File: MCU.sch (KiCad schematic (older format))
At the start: 36 parts, among them P1 CONN_02X05, P2 USB_OTG, SW48 Reset, U1 IS31FL3732, U2 MK20DX256VLH7, X1 CRYSTAL_SMD

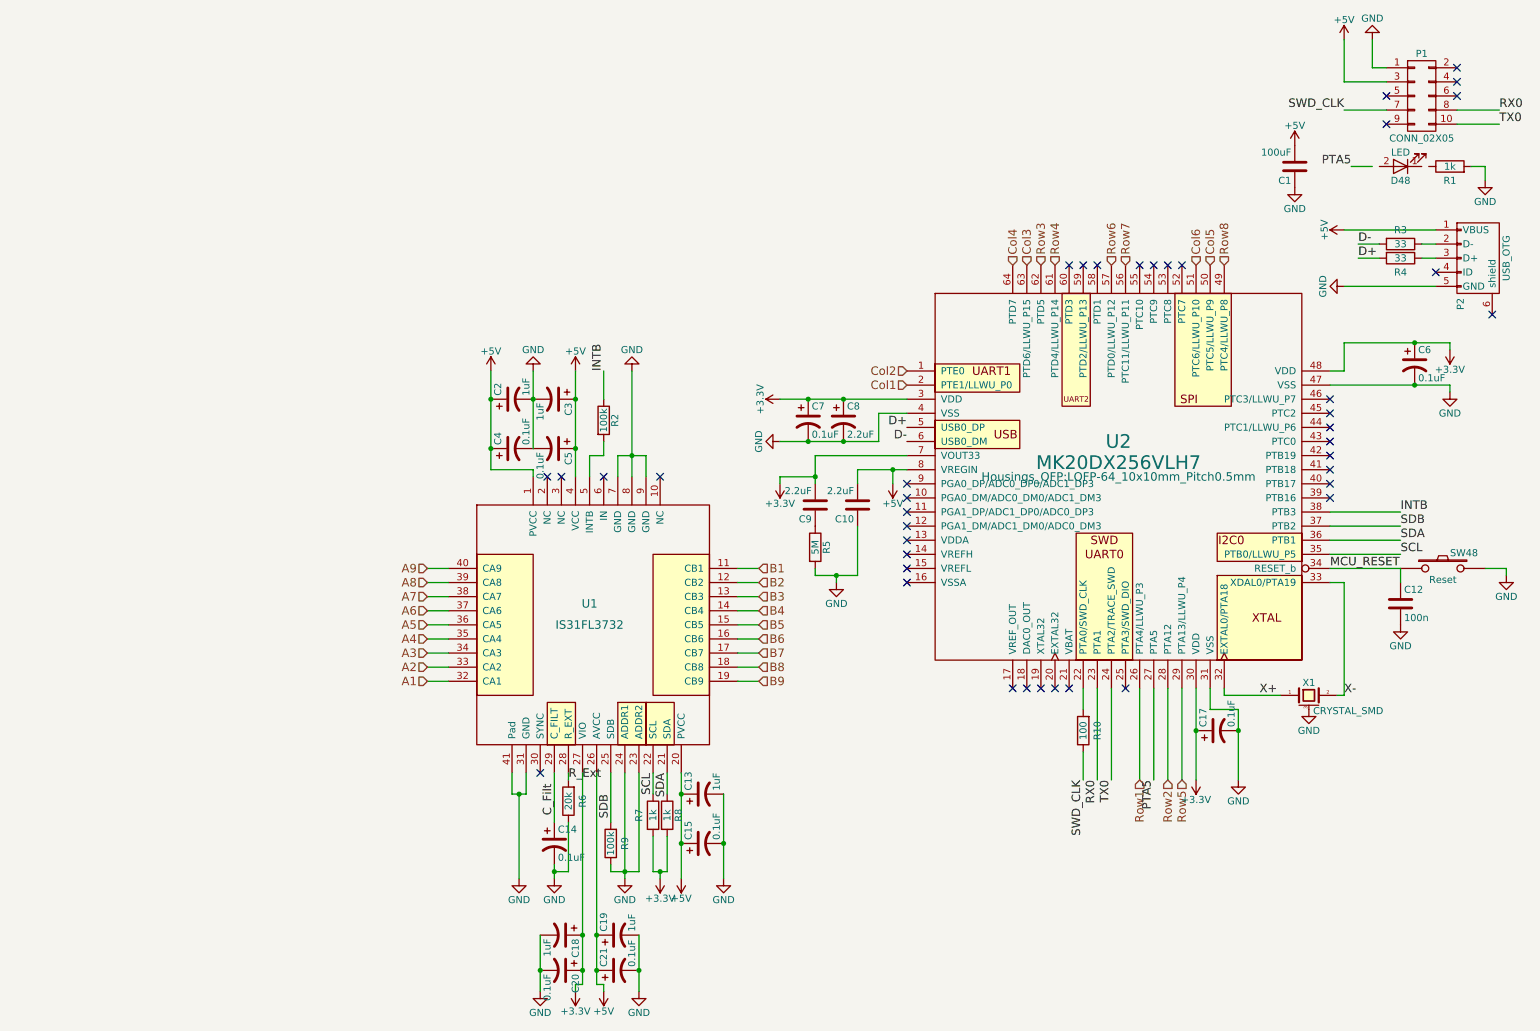
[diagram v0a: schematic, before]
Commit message: Reworked the Board
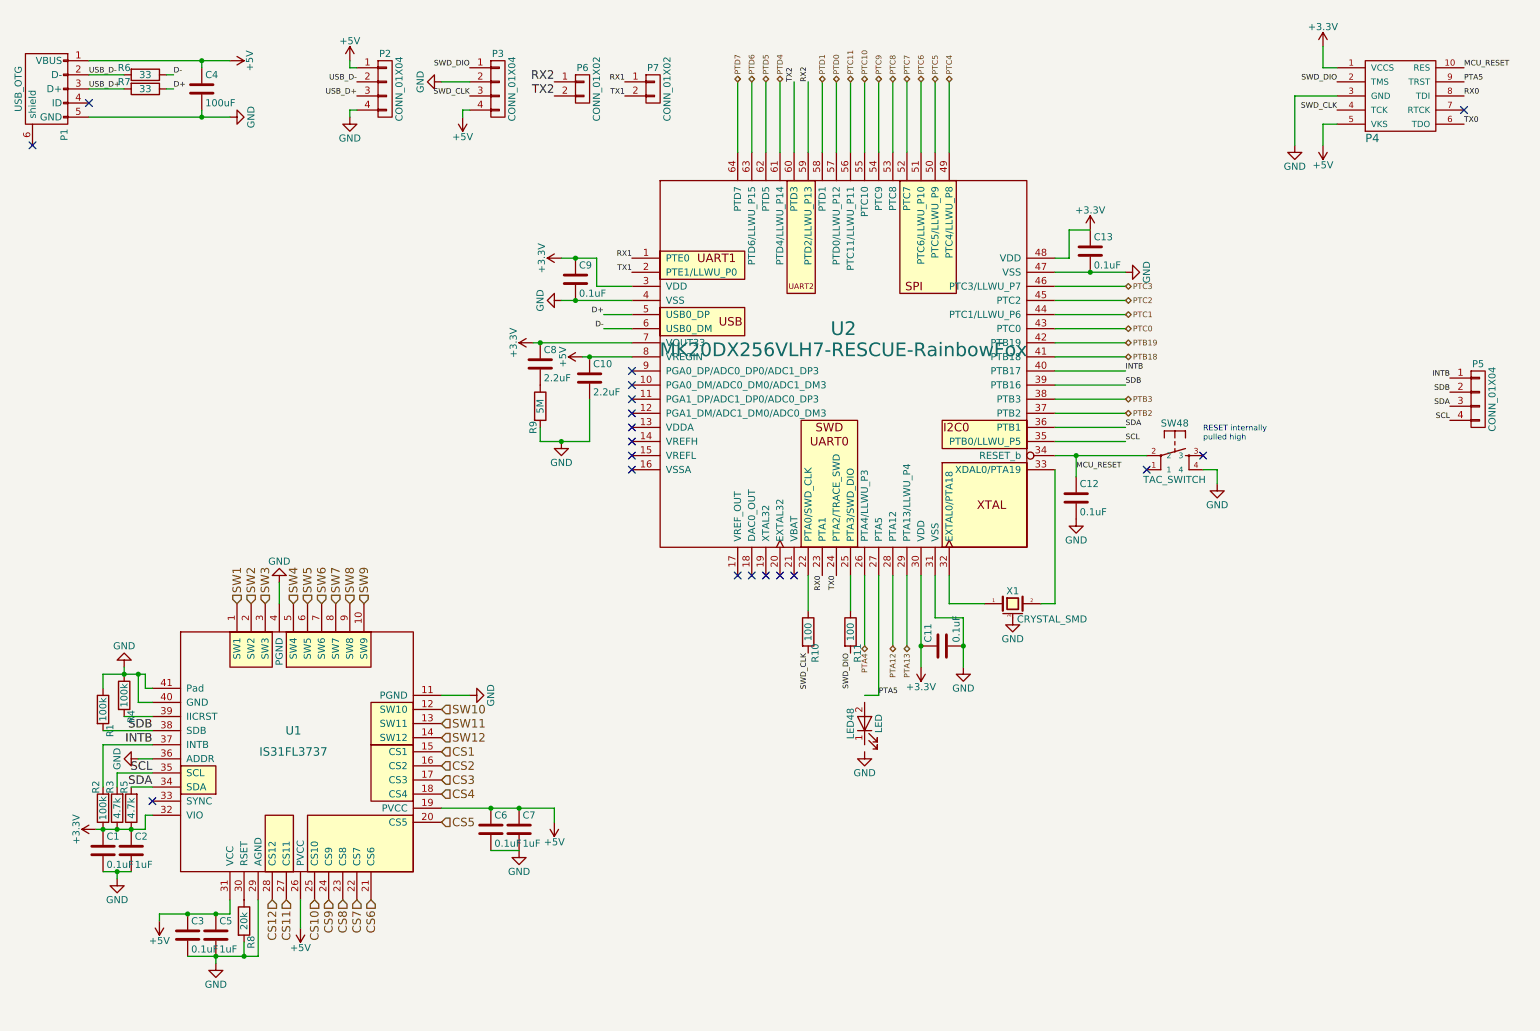
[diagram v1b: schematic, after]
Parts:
- removed C13, C18, C19, C2, C3: 1uF, Capacitors_SMD:C_0603, symbol CP1
- removed C14, C15, C17, C20, C21, C4, C5, C6, C7: 0.1uF, Capacitors_SMD:C_0603, symbol CP1
- removed C8: 2.2uF, Capacitors_SMD:C_0603, symbol CP1
- removed D48: LED, LEDs:LED_0805, symbol LED
- removed P1: CONN_02X05, Pin_Headers:Pin_Header_Straight_2x05, symbol CONN_02X05
- removed P2: USB_OTG, Connect:USB_Micro-B, symbol USB_OTG
- removed SW48: Reset, mx2a:KSEM31GLFS, symbol SW_PUSH
- removed U1: IS31FL3732, Housings_DFN_QFN:UQFN-40-1EP_5x5mm_Pitch0.4mm, symbol IS31FL3732
- removed U2: MK20DX256VLH7, Housings_QFP:LQFP-64_10x10mm_Pitch0.5mm, symbol MK20DX256VLH7
- added C11, C13, C3, C6: 0.1uF, Capacitors_SMD:C_0603, symbol C
- added C2, C5, C7: 1uF, Capacitors_SMD:C_0603, symbol C
- added C4: 100uF, Capacitors_SMD:C_1206, symbol C
- added C8: 2.2uF, Capacitors_SMD:C_0603, symbol C
- added LED48: LED, lib.pretty:LED_0805, symbol LED
- added P1: USB_OTG, lib.pretty:Micro-USB_629105150521, symbol USB_OTG
- added P2, P3, P5: CONN_01X04, lib.pretty:Conn-4, symbol CONN_01X04
- added P4: FLASH_HDR, lib.pretty:JLINK_NEEDLE, symbol FLASH_HDR
- added P6, P7: CONN_01X02, lib.pretty:Conn-2, symbol CONN_01X02
- added R11: 100, Resistors_SMD:R_0603, symbol R
- added SW48: TAC_SWITCH, lib.pretty:PTS810, symbol TAC_SWITCH
- added U1: IS31FL3737, Housings_DFN_QFN:UQFN-40-1EP_5x5mm_Pitch0.4mm, symbol IS31FL3737
- added U2: MK20DX256VLH7-RESCUE-RainbowFox, Housings_QFP:LQFP-64_10x10mm_Pitch0.5mm, symbol MK20DX256VLH7-RESCUE-RainbowFox
- C1: value 100uF -> 0.1uF; footprint Capacitors_SMD:C_0805 -> Capacitors_SMD:C_0603
- C12: value 100n -> 0.1uF
- C9: value 2.2uF -> 0.1uF
- R1: value 1k -> 100k
- R3: value 33 -> 4.7k
- R4: value 33 -> 100k
- R5: value 5M -> 4.7k; footprint Resistors_SMD:R_0805 -> Resistors_SMD:R_0603
- R6: value 20k -> 33
- R7: value 1k -> 33
- R8: value 1k -> 20k
- R9: value 100k -> 5M; footprint Resistors_SMD:R_0603 -> Resistors_SMD:R_0805
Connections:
- net +3V3: now also C1.1, C9.1, R2.1, R3.1, R5.1, C11.1, C13.1, C2.1, C8.1, P4.1 (VCCS), U1.32 (VIO), U2.3 (VDD), U2.30 (VDD), U2.48 (VDD), U2.7 (VOUT33); no longer C9.2, R7.2, R8.2
- net +5V: now also C10.1, C3.1, C4.1, C5.1, C6.1, C7.1, P1.1 (VBUS), P2.1 (P1), P3.4 (P4), P4.5 (VKS), U1.19 (PVCC), U1.26 (PVCC), U1.31 (VCC), U2.8 (VREGIN); no longer C1.2, C10.2
- net D+: now also R7.1, U2.5 (USB0_DP); no longer R4.2
- net D-: now also R6.1, U2.6 (USB0_DM); no longer R3.2
- net GND: now also C1.2, C10.2, C9.2, R1.1, R4.1, R8.2, R9.2, C11.2, C13.2, C2.2, C3.2, C4.2, C5.2, C6.2, C7.2, P1.5 (GND), P2.4 (P4), P3.2 (P2), P4.3 (GND), SW48.4, U1.11 (PGND), U1.29 (AGND), U1.36 (ADDR), U1.4 (PGND), U1.40 (GND), U1.41 (Pad), U2.31 (VSS), U2.4 (VSS), U2.47 (VSS); no longer C1.1, C10.1, R1.2, R5.2, R6.1, R9.1
- net INTB: now also R2.2, P5.1 (P1), U1.37 (INTB), U2.40 (PTB17); no longer R2.1
- net MCU_RESET: now also P4.10 (RES), SW48.2, U2.34 (RESET_b)
- net PTA5: now also P4.9 (TRST), U2.27 (PTA5)
- net RX0: now also P4.8 (TDI), U2.23 (PTA1)
- net SCL: now also R3.2, P5.4 (P4), U1.35 (SCL), U2.35 (PTB0/LLWU_P5); no longer R7.1
- net SDA: now also R5.2, P5.3 (P3), U1.34 (SDA), U2.36 (PTB1); no longer R8.1
- net SDB: now also R1.2, P5.2 (P2), U1.38 (SDB), U2.39 (PTB16); no longer R9.2
- net SWD_CLK: now also R10.2, P3.3 (P3), P4.4 (TCK); no longer R10.1
- net TX0: now also P4.6 (TDO), U2.24 (PTA2/TRACE_SWD)
- net R_Ext renamed USB_D-
- net USB_D-: now also P1.2 (D-), P2.2 (P2)
- net X+: no longer names the net of X1.1
- net X+: now also U2.32 (EXTAL0/PTA18)
- net X-: no longer names the net of X1.2
- net X-: now also U2.33 (XDAL0/PTA19)
- new net: C8.2, R9.1
- new net: R11.1, U2.25 (PTA3/SWD_DIO)
- new net: R10.1, U2.22 (PTA0/SWD_CLK)
- new net: R4.2, U1.39 (IICRST)
- new net: R8.1, U1.30 (RSET)
- new net CS1: U1.15 (CS1)
- new net CS10: U1.25 (CS10)
- new net CS11: U1.27 (CS11)
- new net CS12: U1.28 (CS12)
- new net CS2: U1.16 (CS2)
- new net CS3: U1.17 (CS3)
- new net CS4: U1.18 (CS4)
- new net CS5: U1.20 (CS5)
- new net CS6: U1.21 (CS6)
- new net CS7: U1.22 (CS7)
- new net CS8: U1.23 (CS8)
- new net CS9: U1.24 (CS9)
- new net PTA12: U2.28 (PTA12)
- new net PTA13: U2.29 (PTA13/LLWU_P4)
- new net PTA4: U2.26 (PTA4/LLWU_P3)
- new net PTB18: U2.41 (PTB18)
- new net PTB19: U2.42 (PTB19)
- new net PTB2: U2.37 (PTB2)
- new net PTB3: U2.38 (PTB3)
- new net PTC0: U2.43 (PTC0)
- new net PTC1: U2.44 (PTC1/LLWU_P6)
- new net PTC10: U2.55 (PTC10)
- new net PTC11: U2.56 (PTC11/LLWU_P11)
- new net PTC2: U2.45 (PTC2)
- new net PTC3: U2.46 (PTC3/LLWU_P7)
- new net PTC4: U2.49 (PTC4/LLWU_P8)
- new net PTC5: U2.50 (PTC5/LLWU_P9)
- new net PTC6: U2.51 (PTC6/LLWU_P10)
- new net PTC7: U2.52 (PTC7)
- new net PTC8: U2.53 (PTC8)
- new net PTC9: U2.54 (PTC9)
- new net PTD0: U2.57 (PTD0/LLWU_P12)
- new net PTD1: U2.58 (PTD1)
- new net PTD4: U2.61 (PTD4/LLWU_P14)
- new net PTD5: U2.62 (PTD5)
- new net PTD6: U2.63 (PTD6/LLWU_P15)
- new net PTD7: U2.64 (PTD7)
- new net RX1: P7.1 (P1), U2.1 (PTE0)
- new net RX2: P6.1 (P1), U2.59 (PTD2/LLWU_P13)
- new net SW1: U1.1 (SW1)
- new net SW10: U1.12 (SW10)
- new net SW11: U1.13 (SW11)
- new net SW12: U1.14 (SW12)
- new net SW2: U1.2 (SW2)
- new net SW3: U1.3 (SW3)
- new net SW4: U1.5 (SW4)
- new net SW5: U1.6 (SW5)
- new net SW6: U1.7 (SW6)
- new net SW7: U1.8 (SW7)
- new net SW8: U1.9 (SW8)
- new net SW9: U1.10 (SW9)
- new net SWD_DIO: P3.1 (P1), P4.2 (TMS), R11.2
- new net TX1: P7.2 (P2), U2.2 (PTE1/LLWU_P0)
- new net TX2: P6.2 (P2), U2.60 (PTD3)
- new net USB_D+: P1.3 (D+), P2.3 (P3), R7.2
- no-connect marks 41 -> 19
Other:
- note added: "RESET internally\npulled high"
